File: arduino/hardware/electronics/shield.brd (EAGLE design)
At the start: 101.6 x 53 mm, 22 parts

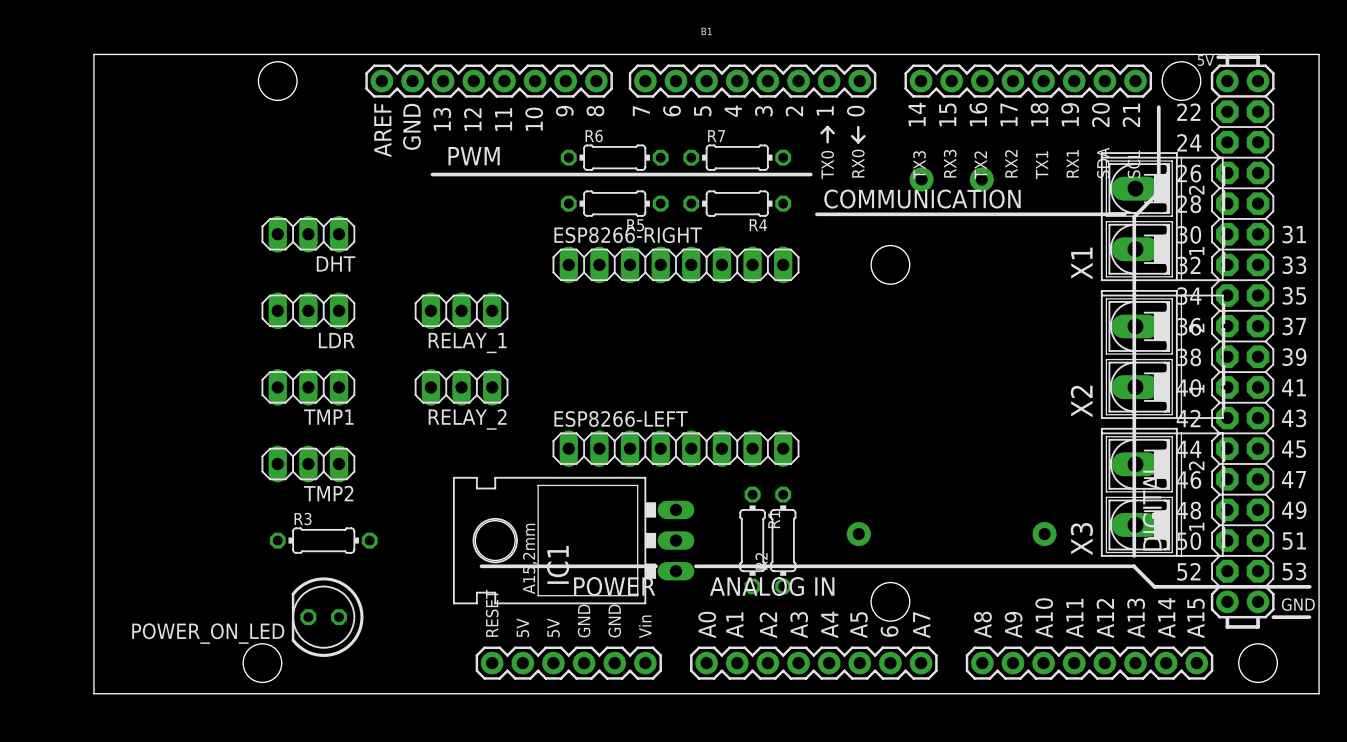
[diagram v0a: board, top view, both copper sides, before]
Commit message: Updated electronics
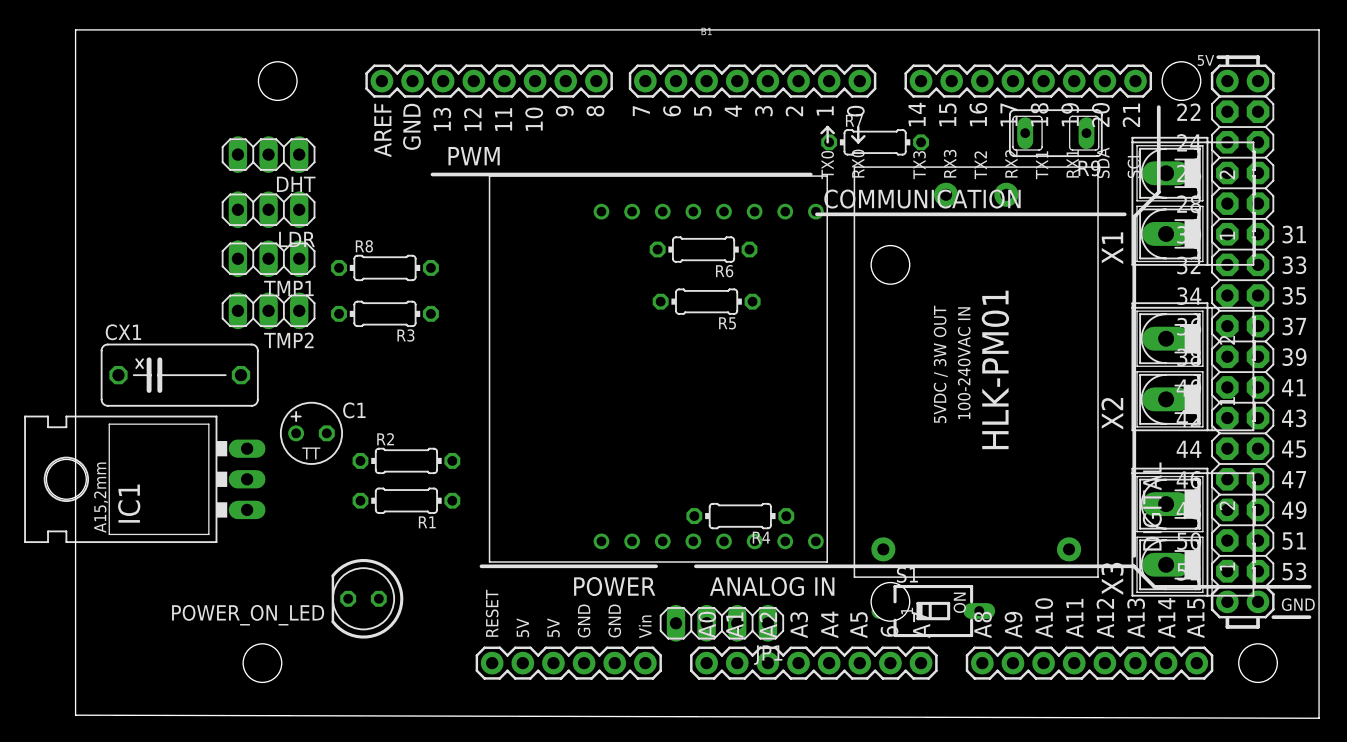
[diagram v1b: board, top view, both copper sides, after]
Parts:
- removed ESP8266-LEFT, ESP8266-RIGHT: (no value), pinhead:1X08
- removed RELAY_1, RELAY_2: (no value), pinhead:1X03
- added C1: 1uf, rcl:TT2D5
- added CX1: 0.1uF, resistor:XC10B5
- added JP1: (no value), pinhead:1X04
- added R8: 4.7k, eagle-ltspice:0204/7
- added R9: S2220, varistor:S2220
- added S1: (no value), switch-dil:SD4-01
- added U$4: ESP8266_SHIELD, esp8266_shield:ESP8266_SHIELD
- IC1: value (none) -> 3.3V
- moved IC1 35.9 mm to (40.6, 43.2)
- moved R2 31.9 mm to (57.7, 44.7), turned to 0 degrees
- moved R1 28.9 mm to (57.7, 41.4), turned to 180 degrees
- moved R4 25.9 mm to (85.3, 40.1)
- moved R3 19.5 mm to (55.9, 56.9), turned to 180 degrees
- moved TMP2 13.1 mm to (46.2, 57.1)
- moved R7 11.5 mm to (96.5, 71.1)
- moved TMP1 11.2 mm to (46.2, 61.5)
- moved R5 11.1 mm to (82.5, 57.9)
- moved R6 10.6 mm to (82.3, 62.2), turned to 180 degrees
- moved LDR 9.01 mm to (46.2, 65.5)
- moved DHT 7.38 mm to (46.2, 70.1)
- moved X3 4.17 mm to (120.7, 38.6)
- moved POWER_ON_LED 3.64 mm to (54.1, 33.3)
- moved X1 2.84 mm to (120.7, 66.0)
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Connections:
- removed net ESP8266_CH_PD: ESP8266-LEFT.3, R4.2
- removed net ESP_8266_TX: B1.15
- removed net N$1: U$1.AC1, X1.1, X2.1, X3.1
- new net DC+: S1.2, U$1.DC+
- new net GND4: B1.GND@4, DHT.2, LDR.2, TMP1.2, TMP2.2
- new net N$10: R9.2, U$1.AC1, X1.1, X2.1, X3.1
- new net N$19: R4.2, U$4.CH_PD
- net 5V: now also R8.2
- net ESP8266_TX: now also B1.15, U$4.TXD; no longer ESP8266-RIGHT.1
- net GND0: no longer DHT.2, LDR.2, TMP1.2, TMP2.2
- net GND1: now also C1.-, CX1.2, JP1.4, U$4.GND; no longer ESP8266-RIGHT.8, RELAY_1.2, RELAY_2.2
- net N$2: now also R9.1
- net N$8: now also U$4.RXD; no longer ESP8266-RIGHT.2
- net POWER_SUPPLY_3.3V: now also C1.+, U$4.VCC; no longer ESP8266-LEFT.8
- net POWER_SUPPLY_5V: now also CX1.1, JP1.1, S1.1; no longer RELAY_1.3, RELAY_2.3, U$1.DC+
- net RELAY_1: now also B1.A1, JP1.2; no longer RELAY_1.1
- net RELAY_2: now also B1.A0, JP1.3; no longer RELAY_2.1
- net TMP: now also R8.1
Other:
- board size 101.6 x 53 mm -> 103.1 x 57.1 mm
